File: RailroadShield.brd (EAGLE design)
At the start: 88.9 x 50.8 mm, 37 parts, among them J4 RJ45-8X, J5 RJ45-8X, J6 RJ12, J7 RJ12, Q1 2N3904, U1 LM393N, U2 MCP2515-P, U3 MCP2551-P, U4 LM317LD, Y1 16Mhz

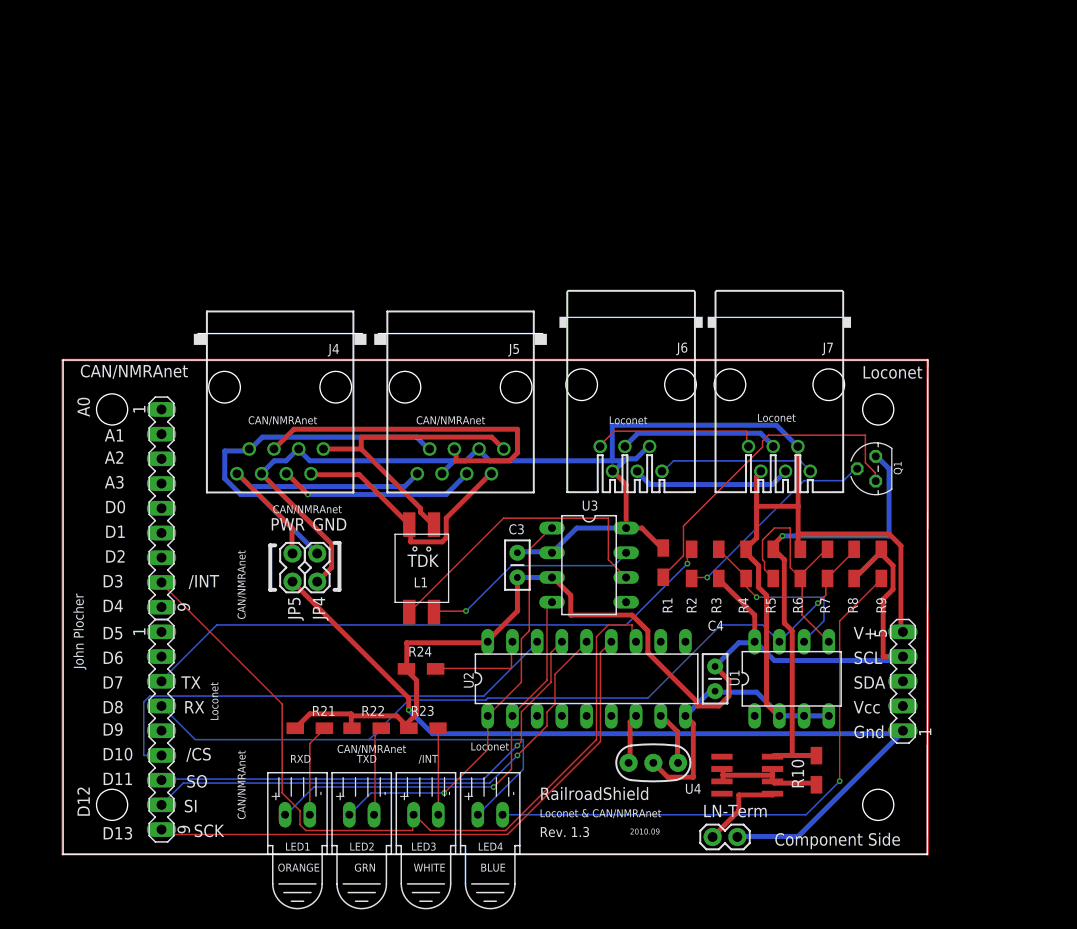
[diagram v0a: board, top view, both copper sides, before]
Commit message: 2.0
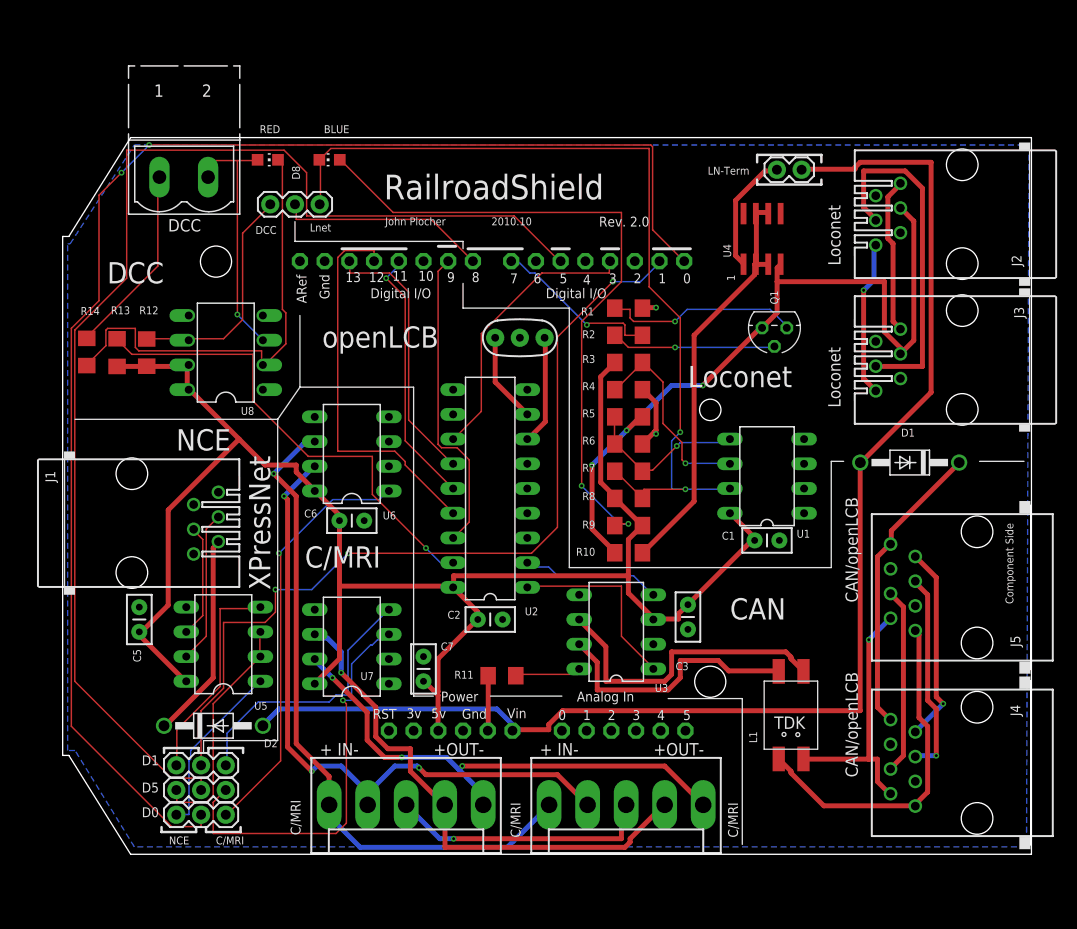
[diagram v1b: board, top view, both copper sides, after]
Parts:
- removed C4: 0.1uf, SparkFun:CAP-PTH-SMALL2
- removed J6, J7: RJ12, con-amp:520250-3
- removed JP4: (no value), SparkFun:1X02_LOCK
- removed LED1, LED2, LED3: (no value), MCP:Q62902-B155
- removed R21, R22, R23: 470R, rcl:R1206W
- removed R24: 10k, rcl:R1206W
- removed SV2: (no value), con-lstb:MA05-1
- added C1, C2: .1uf, SparkFun:CAP-PTH-SMALL2
- added C5, C6, C7: .1uF, SparkFun:CAP-PTH-SMALL2
- added D1, D2: 1N4004, diode:DO41-10
- added J1: RJ12, con-amp:520250-3
- added JP2: RXD-LN, SparkFun:1X03
- added JP6: EN, SparkFun:1X03
- added JP7: TXD, SparkFun:1X03
- added LED5: DCC, MCP:CHIP-LED0805
- added MOD1: ARDUINO DUEMILANOVE, microbuilder:ARDUINO-BIGSHIELD
- added R11: 100k, rcl:R1206
- added R12: 10K, SparkFun:1206
- added R13: 10k, rcl:R1206
- added R14: 1K, SparkFun:1206
- added U5, U6, U7: MAX3468CPA, maxim:DIL08
- added U8: 6N137, optocoupler:DIL08
- added X1, X2: 5-pin Molex, con-molex:KK-156-5
- added X3: (no value), con-phoenix-500:MSTBV2
- C3: value 0.1uf -> .1uf
- J2, J3: value (none) -> RJ12; device con-lstb:MA09-1 -> con-amp:520250-3
- J4, J5: value RJ45-8X -> RJ45
- JP1: value (none) -> LN_TERM
- JP5: value (none) -> RXD; device SparkFun:1X02_LOCK -> SparkFun:1X03
- LED4: value (none) -> Loconet; device MCP:Q62902-B155 -> MCP:CHIP-LED0805
- R1: value 47R -> 15R; device rcl:R1206W -> rcl:R1206
- R10, R2, R3, R4, R5, R6, R7, R8, R9: device rcl:R1206W -> rcl:R1206
- moved J3 90.7 mm to (92.5, 50.8), turned to 90 degrees
- moved J2 87.7 mm to (92.5, 65.8), turned to 90 degrees
- moved J4 81.4 mm to (94.0, 9.40), turned to 90 degrees
- moved LED4 76.7 mm to (27.4, 71.4)
- moved JP1 68.9 mm to (73.4, 70.4)
- moved J5 56.9 mm to (94.0, 27.4), turned to 90 degrees
- moved U4 55.1 mm to (71.9, 63.2), turned to 0 degrees
- moved Y1 45.8 mm to (47.0, 53.1), turned to 180 degrees
- moved L1 40.4 mm to (74.7, 14.5), turned to 90 degrees
- moved R10 29.5 mm to (58.2, 31.0), turned to 180 degrees
- moved JP5 27.5 mm to (16.8, 4.06), turned to 180 degrees
- moved R1 26.4 mm to (58.2, 56.1), turned to 180 degrees
- moved R9 26.3 mm to (58.2, 33.8), turned to 0 degrees
- moved R2 24.4 mm to (58.2, 53.3), turned to 0 degrees
- moved R8 24.1 mm to (58.2, 36.6), turned to 0 degrees
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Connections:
- removed net A0: J2.1
- removed net A1: J2.2
- removed net A2: J2.3
- removed net A3: J2.4
- removed net D10: J3.6, U2.16
- removed net D2: J2.7
- removed net D4: J2.9
- removed net D6: J3.2
- removed net N$12: LED2.K, R22.1
- removed net N$14: LED3.K, R23.1
- removed net PWR-: J4.7, J5.7, JP4.1
- new net -OUT+: U7.7, X1.1, X2.1
- new net 3V: MOD1.3V
- new net CMRIRX: JP5.1, U6.1
- new net CMRITX: JP7.1, U7.4
- new net CMRITXEN: JP6.1, U7.3
- new net DCCRX: JP2.1, R12.1, U8.6
- new net IN+: U6.6, X1.5, X2.5
- new net IN-: U6.7, X1.4, X2.4
- new net LNRX: JP2.3, LED4.C, R7.2, R8.2, U1.7
- new net N$20: R14.1, X3.1
- new net N$23: J2.3, J3.3
- new net N$24: J1.4, U5.6
- new net N$25: J1.3, U5.7
- new net N$26: D2.C, J1.5
- new net N$4: R11.1, U3.8
- new net NCERX: JP5.3, U5.1
- new net NCETX: JP7.3, U5.4
- new net NCETXEN: JP6.3, U5.2, U5.3
- new net OUT+: U7.6, X1.2, X2.2
- new net SHIELD: X1.3, X2.3
- net /RESET: now also R13.1; no longer R24.1
- net D0: now also JP5.2, MOD1.D0; no longer J2.5
- net D1: now also JP7.2, MOD1.D1; no longer J2.6
- net D11: now also MOD1.D11, U2.14; no longer J3.7, U2.15
- net D12: now also MOD1.D12, U2.15; no longer J3.8, U2.14
- net D13: now also MOD1.D13; no longer J3.9
- net D3: now also MOD1.D3; no longer J2.8, LED3.A
- net D5: now also JP6.2, MOD1.D5; no longer J3.1
- net D7: now also MOD1.D7; no longer J3.3
- net D8: now also JP2.2, MOD1.D8; no longer J3.4, LED4.A, R7.2, R8.2, U1.7
- net D9: now also MOD1.D9, U2.16; no longer J3.5
- net GND: now also C1.2, C2.2, C5.2, C6.2, C7.2, J1.2, J2.2, J2.5, J3.2, J3.5, MOD1.GND, MOD1.GND1, MOD1.GND2, R11.2, U5.5, U6.2, U6.3, U6.4, U6.5, U7.2, U7.5, U8.5; no longer C4.2, J6.2, J6.5, J7.2, J7.5, JP4.2, SV2.5, U3.8
- net LOCONET: now also J2.4, J3.4
- net N$10: now also J2.6, J3.6; no longer J6.6, J7.6
- net N$11: now also J4.7, J5.7; no longer LED1.K, R21.1
- net N$13: now also LED5.A, U8.3, X3.2; no longer J6.3, J7.3
- net N$15: now also LED4.A; no longer LED4.K
- net N$16: now also LED5.C, R14.2, U8.2; no longer J6.4, J7.4
- net N$9: now also J2.1, J3.1; no longer J6.1, J7.1
- net PWR+: now also D1.C; no longer JP5.1
- net RXCAN: no longer LED1.A
- net TXCAN: no longer LED2.A
- net V+: now also D1.A, D2.A, MOD1.VIN; no longer JP5.2, SV2.1
- net VCC: now also C1.1, C2.1, C5.1, C6.1, C7.1, MOD1.5V, R12.2, R13.2, U5.8, U6.8, U7.8, U8.7, U8.8; no longer C4.1, R21.2, R22.2, R23.2, R24.2, SV2.4
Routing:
- net N$4: track 279.4 -> 7.18 mm
- net GND: track 198.7 -> 14.1 mm, vias 0 -> 2
- net D0: track 0.00 -> 146.8 mm, vias 0 -> 2
- net D5: track 0.00 -> 127.0 mm
- net LNRX: track 0.00 -> 91.1 mm, vias 0 -> 2
- net D1: track 0.00 -> 88.7 mm, vias 0 -> 3
- net D8: track 108.7 -> 21.5 mm, vias 1 -> 0
- net IN+: track 0.00 -> 68.9 mm, vias 0 -> 1
- net IN-: track 0.00 -> 68.9 mm, vias 0 -> 3
- net VCC: track 121.8 -> 179.9 mm
- net D3: track 84.3 -> 29.0 mm
- net OUT+: track 0.00 -> 53.9 mm, vias 0 -> 1
- net -OUT+: track 0.00 -> 52.8 mm, vias 0 -> 3
- net D10: track 50.4 -> 0.00 mm
- net V+: track 91.6 -> 137.8 mm, vias 1 -> 0
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- added copper zone on layer 16, net GND
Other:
- board size 88.9 x 50.8 mm -> 99.6 x 73.7 mm
- board text added: "+ IN-"
- board text added: "+OUT-"
- board text added: ".com"
- board text added: "1"
- board text added: "2010.10"
- board text added: "C/MRI"
- board text added: "CAN"
- board text added: "CAN/openLCB"
- board text added: "DCC"
- board text added: "Lnet"
- board text added: "Model Railroading is fun!"
- board text added: "NCE"
- board text added: "RED"
- board text added: "Railroadshield"
- board text added: "Rev. 2.0"
- board text added: "SP Coast"
- board text added: "XPressNet"
- board text added: "interface board"
- board text added: "openLCB"
- board text added: "www."
- board text removed: "/CS"
- board text removed: "/INT"
- board text removed: "2010.09"
- board text removed: "A0"
- board text removed: "A1"
- board text removed: "A2"
- board text removed: "A3"
- board text removed: "CAN/NMRAnet"
- board text removed: "D10"
- board text removed: "D11"
- board text removed: "D12"
- board text removed: "D13"
- board text removed: "D2"
- board text removed: "D3"
- board text removed: "D4"
- board text removed: "D6"
- board text removed: "D7"
- board text removed: "D9"
- board text removed: "GND"
- board text removed: "GRN"
- board text removed: "Gnd"
- board text removed: "Loconet & CAN/NMRAnet"
- board text removed: "ORANGE"
- board text removed: "PWR"
- board text removed: "RX"
- board text removed: "RXD"
- board text removed: "Rev. 1.3"
- board text removed: "SCK"
- board text removed: "SCL"
- board text removed: "SDA"
- board text removed: "SI"
- board text removed: "SO"
- board text removed: "TX"
- board text removed: "TXD"
- board text removed: "V+"
- board text removed: "Vcc"
- board text removed: "WHITE"

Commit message: 2.1
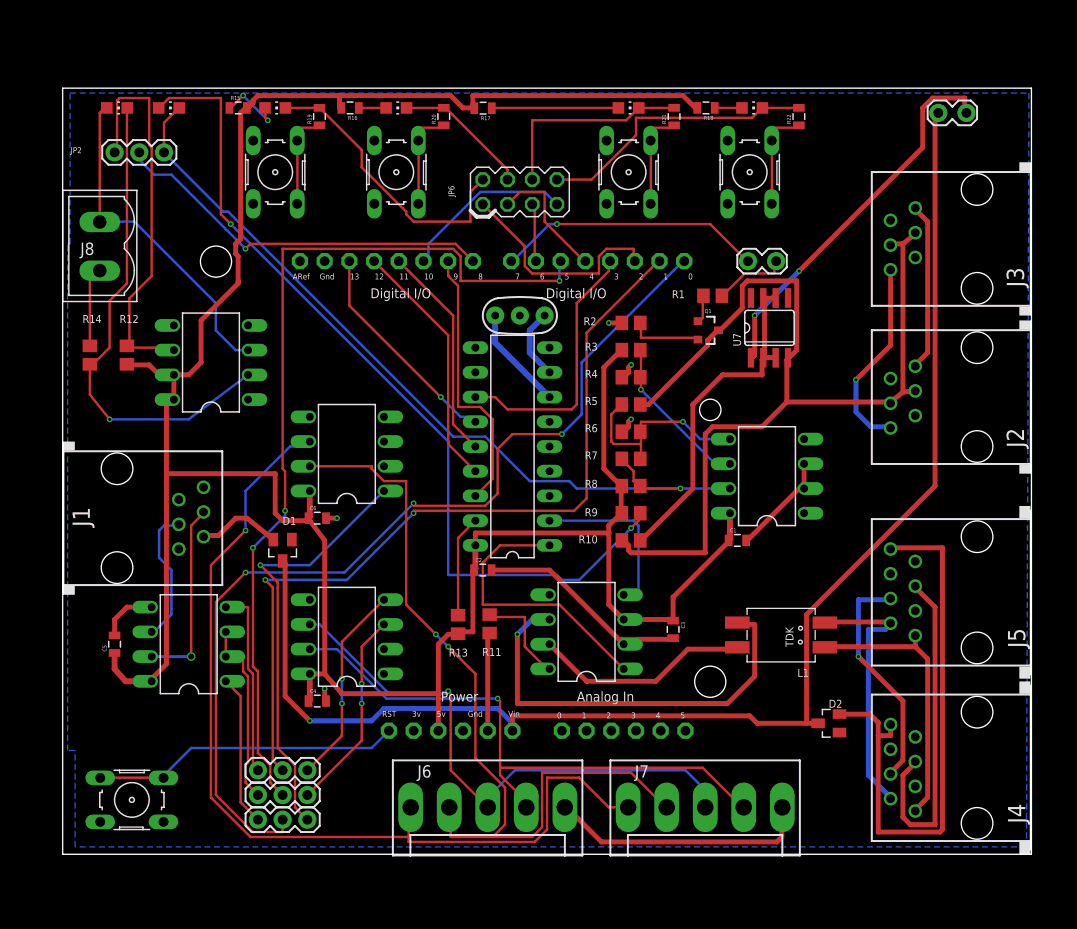
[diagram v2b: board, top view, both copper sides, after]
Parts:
- removed C7: .1uF, SparkFun:CAP-PTH-SMALL2
- removed MOD1: ARDUINO DUEMILANOVE, microbuilder:ARDUINO-BIGSHIELD
- removed X1, X2: 5-pin Molex, con-molex:KK-156-5
- removed X3: (no value), con-phoenix-500:MSTBV2
- added C4: 0.01uf, MCP:0805
- added J6, J7: KK-156-5, MCP:KK-156-5
- added J8: MSTB-02, MCP:MSTBV2
- added JP3: RxD, MCP:1X03
- added JP4: EN, MCP:1X03
- added LED1: Blue, MCP:CHIP-LED0805
- added LED2: Gold, MCP:CHIP-LED0805
- added LED3: Green, MCP:CHIP-LED0805
- added LED6: Loconet, MCP:CHIP-LED0805
- added R15, R16, R17, R18, R19, R20, R21, R22: 660R, MCP:0805
- added S1, S2, S3, S4: B3F-1052, MCP:B3F-10XX
- added S5: B3F-1000, MCP:B3F-10XX
- added U$1: ARDUINODUEMILANOVE, MCP:ARDUINO-BIGSHIELD
- C1, C2, C3: value .1uf -> 0.01uf; device SparkFun:CAP-PTH-SMALL2 -> MCP:0805
- C5, C6: value .1uF -> 0.01uf; device SparkFun:CAP-PTH-SMALL2 -> MCP:0805
- D1, D2: value 1N4004 -> BAV199; device diode:DO41-10 -> diode:SOT23
- J1, J2, J3: value RJ12 -> 5520250-3; device con-amp:520250-3 -> MCP:RJ11-NO_SHIELD
- J4, J5: value RJ45 -> 5520426-4; device con-tycoelectronics:RJ45-NO-SHIELD -> MCP:RJ45-NO-SHIELD
- JP1: value LN_TERM -> LN-TERM; device SparkFun:1X02 -> MCP:1X02_LOCK
- JP2: device SparkFun:1X03 -> MCP:1X03
- JP5: value RXD -> TxD; device SparkFun:1X03 -> MCP:1X03
- JP6: value EN -> MA04-2; device SparkFun:1X03 -> MCP:MA04-2
- JP7: value TXD -> LNTX; device SparkFun:1X03 -> MCP:1X02_LOCK
- LED4: value Loconet -> Green
- Q1: value 2N3904 -> PMBT2222; device transistor:TO92 -> MCP:SOT23-3
- R1: value 15R -> 4k7; device rcl:R1206 -> rcl:R0805
- R10, R11, R13, R3, R4, R5, R6, R7, R8: device rcl:R1206 -> rcl:R0805
- R12: device SparkFun:1206 -> rcl:R0805
- R14: value 1K -> 1k; device SparkFun:1206 -> rcl:R0805
- R2: value 4k7 -> 18R; device rcl:R1206 -> rcl:R0805
- R9: value 470R -> 1k; device rcl:R1206 -> rcl:R0805
- U4: value LM317LD -> MAX3468CPA; device linear:SO08 -> MCP:DIL08
- U5, U6: device maxim:DIL08 -> MCP:DIL08
- U7: value MAX3468CPA -> LM317LD; device maxim:DIL08 -> MCP:SO08
- Y1: device SparkFun:RESONATOR-PTH -> MCP:RESONATOR-PTH
- moved JP7 76.6 mm to (73.2, 61.0)
- moved JP6 68.5 mm to (47.0, 68.1), turned to 0 degrees
- moved D1 65.1 mm to (22.6, 31.2)
- moved D2 63.2 mm to (78.7, 13.5), turned to 90 degrees
- moved U4 59.1 mm to (29.2, 22.4), turned to 90 degrees
- moved U7 54.0 mm to (72.6, 54.1), turned to 0 degrees
- moved R13 44.8 mm to (40.6, 23.6)
- moved LED4 43.8 mm to (70.9, 76.7), turned to 270 degrees
- moved JP1 20.2 mm to (92.7, 76.2), turned to 180 degrees
- moved J2 18.9 mm to (94.0, 47.0)
- moved JP2 16.9 mm to (5.33, 72.1)
- moved LED5 16.4 mm to (5.59, 76.7)
- moved J3 12.5 mm to (94.0, 63.2)
- moved JP5 9.55 mm to (25.1, 8.64)
- moved R1 8.73 mm to (66.8, 57.4)
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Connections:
- net N$10 renamed RAILSYNCA
- net N$16 renamed DCC-A
- net N$18 renamed O-RESA
- net N$21 renamed O-RESB
- net N$24 renamed N-A
- net N$25 renamed N-B
- net N$4 renamed RS
- net N$9 renamed RAILSYNCB
- net OSC1 renamed N$12
- removed net -OUT+: U7.7, X1.1, X2.1
- removed net IN+: U6.6, X1.5, X2.5
- removed net IN-: U6.7, X1.4, X2.4
- removed net N$13 (its old number): LED5.A, U8.3, X3.2
- removed net N$15: LED4.A, R9.1
- removed net N$17: R10.1, U4.2, U4.3, U4.6, U4.7
- removed net N$19: JP1.1, U4.1
- removed net N$20: R14.1, X3.1
- removed net N$23: J2.3, J3.3
- removed net N$26: D2.C, J1.5
- removed net OUT+: U7.6, X1.2, X2.2
- removed net PWR+: D1.C, J4.8, J5.8
- removed net SHIELD: X1.3, X2.3
- new net A/RESET: S5.1, S5.2, U$1.RESET
- new net CAN-H: J4.1, J5.1, L1.3
- new net CAN-L: J4.2, J5.2, L1.4
- new net CAN-PWR+: D2.2, J4.8, J5.8
- new net D10: JP6.7, U$1.D10
- new net D2: JP6.1, U$1.D2
- new net D4: JP6.3, U$1.D4
- new net D6: JP6.5, U$1.D6
- new net DCCB: J8.2, LED5.A, U8.3
- new net IO1: JP6.2, LED1.C, R19.2
- new net IO2: JP6.4, LED2.C, R20.2
- new net IO3: JP6.6, LED3.C, R21.2
- new net IO4: JP6.8, LED4.C, R22.2
- new net L6+: LED6.A, R9.2
- new net LN-TX: Q1.1, R1.2
- new net LNTX: JP7.1, R1.1
- new net LOCONET-IN: R5.2, R6.1, R7.1, U1.5
- new net N$10: J6.5, J7.5, U6.6
- new net N$4: LED4.A, R18.1
- new net N$8: J6.3, J7.3, U4.6
- new net N$9: J6.4, J7.4, U6.7
- new net NCE-PWR+: D1.2, J1.5
- new net S1+: R19.1, S1.3, S1.4
- new net S2+: R20.1, S2.3, S2.4
- new net S3+: R21.1, S3.3, S3.4
- new net S4+: R22.1, S4.3, S4.4
- new net TERM-PWR: JP1.1, U7.1
- new net V-LNREF: R3.2, R4.1, U1.6
- new net VOUT: R10.1, U7.2, U7.3, U7.6, U7.7
- net 3V: now also U$1.3V; no longer MOD1.3V
- net CANH: now also L1.2, U3.7; no longer J4.1, J5.1, L1.3
- net CANL: now also L1.1, U3.6; no longer J4.2, J5.2, L1.4
- net CMRIRX: now also JP3.1; no longer JP5.1
- net CMRITX: now also JP5.1, U4.4; no longer JP7.1, U7.4
- net CMRITXEN: now also JP4.1, U4.3; no longer JP6.1, U7.3
- net D0: now also JP3.2, U$1.D0; no longer JP5.2, MOD1.D0
- net D1: now also JP5.2, U$1.D1; no longer JP7.2, MOD1.D1
- net D11: now also U$1.D11; no longer MOD1.D11
- net D12: now also U$1.D12; no longer MOD1.D12
- net D13: now also U$1.D13; no longer MOD1.D13
- net D3: now also U$1.D3; no longer MOD1.D3
- net D5: now also JP4.2, U$1.D5; no longer JP6.2, MOD1.D5
- net D7: now also JP7.2, U$1.D7; no longer MOD1.D7, R2.2
- net D8: now also U$1.D8; no longer MOD1.D8
- net D9: now also U$1.D9; no longer MOD1.D9
- net GND: now also C4.2, J4.7, J5.7, R2.2, R4.2, R6.2, S1.1, S1.2, S2.1, S2.2, S3.1, S3.2, S4.1, S4.2, S5.3, S5.4, U$1.GND, U$1.GND1, U$1.GND2, U4.2, U4.5; no longer C7.2, MOD1.GND, MOD1.GND1, MOD1.GND2, R1.1, R4.1, R6.1, U7.2, U7.5
- net LNRX: now also LED6.C; no longer LED4.C
- net LOCONET: now also J2.3, J3.3, Q1.3, U7.4; no longer Q1.1, U4.4
- net N$11: now also J8.1, R14.1; no longer J4.7, J5.7
- net N$2: now also LED2.A, R16.1; no longer R5.2, R6.2, R7.1, U1.5
- net N$3: now also LED3.A, R17.1; no longer L1.1, U3.6
- net N$5: now also LED1.A, R15.1; no longer R3.2, R4.2, U1.6
- net N$6: now also J6.1, J7.1; no longer Q1.3, R1.2
- net N$7: now also J6.2, J7.2, U4.7; no longer L1.2, U3.7
- net NCERX: now also JP3.3; no longer JP5.3
- net NCETX: now also JP5.3; no longer JP7.3
- net NCETXEN: now also JP4.3; no longer JP6.3
- net V+: now also D1.3, D2.3, U$1.VIN; no longer D1.A, D2.A, MOD1.VIN
- net VCC: now also C4.1, R15.2, R16.2, R17.2, R18.2, R9.1, U$1.5V, U4.8; no longer C7.1, MOD1.5V, R9.2, U7.8
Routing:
- net N$10: track 0.00 -> 97.1 mm, vias 0 -> 1
- net L6+: track 0.00 -> 88.7 mm, vias 0 -> 2
- net VCC: track 179.9 -> 268.5 mm
- net N$9: track 0.00 -> 84.9 mm, vias 0 -> 2
- net N$15: track 69.0 -> 0.00 mm, vias 2 -> 0
- net IN+: track 68.9 -> 0.00 mm, vias 1 -> 0
- net IN-: track 68.9 -> 0.00 mm, vias 3 -> 0
- net CAN-PWR+: track 0.00 -> 59.1 mm
- net N$8: track 0.00 -> 58.3 mm, vias 0 -> 1
- net OUT+: track 53.9 -> 0.00 mm, vias 1 -> 0
- net -OUT+: track 52.8 -> 0.00 mm, vias 3 -> 0
- net D0: track 146.8 -> 98.3 mm, vias 2 -> 3
- net GND: track 14.1 -> 56.9 mm, vias 2 -> 5
- net N$17: track 42.4 -> 0.00 mm
- net TERM-PWR: track 0.00 -> 39.5 mm, vias 0 -> 2
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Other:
- board size 99.6 x 73.7 mm -> 99.6 x 78.7 mm
- board text added: ""Go Bears!""
- board text added: "15mA Loconet Termination"
- board text added: "2"
- board text added: "2012.03"
- board text added: "3"
- board text added: "4"
- board text added: "D10"
- board text added: "D2"
- board text added: "D4"
- board text added: "D6"
- board text added: "D7"
- board text added: "Go Bears!"
- board text added: "I/O"
- board text added: "Reset"
- board text added: "Rev. 2.1"
- board text added: "Shield"
- board text added: "So then it's up with the Blue and Gold, Down with the Red..."
- board text added: "layout interface board"
- board text removed: "2010.10"
- board text removed: "BLUE"
- board text removed: "LN-Term"
- board text removed: "Lnet"
- board text removed: "RED"
- board text removed: "Rev. 2.0"
- board text removed: "interface board"
